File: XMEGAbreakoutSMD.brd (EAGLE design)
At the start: 160 x 100 mm, 23 parts, among them IC1 XMEGA16A4

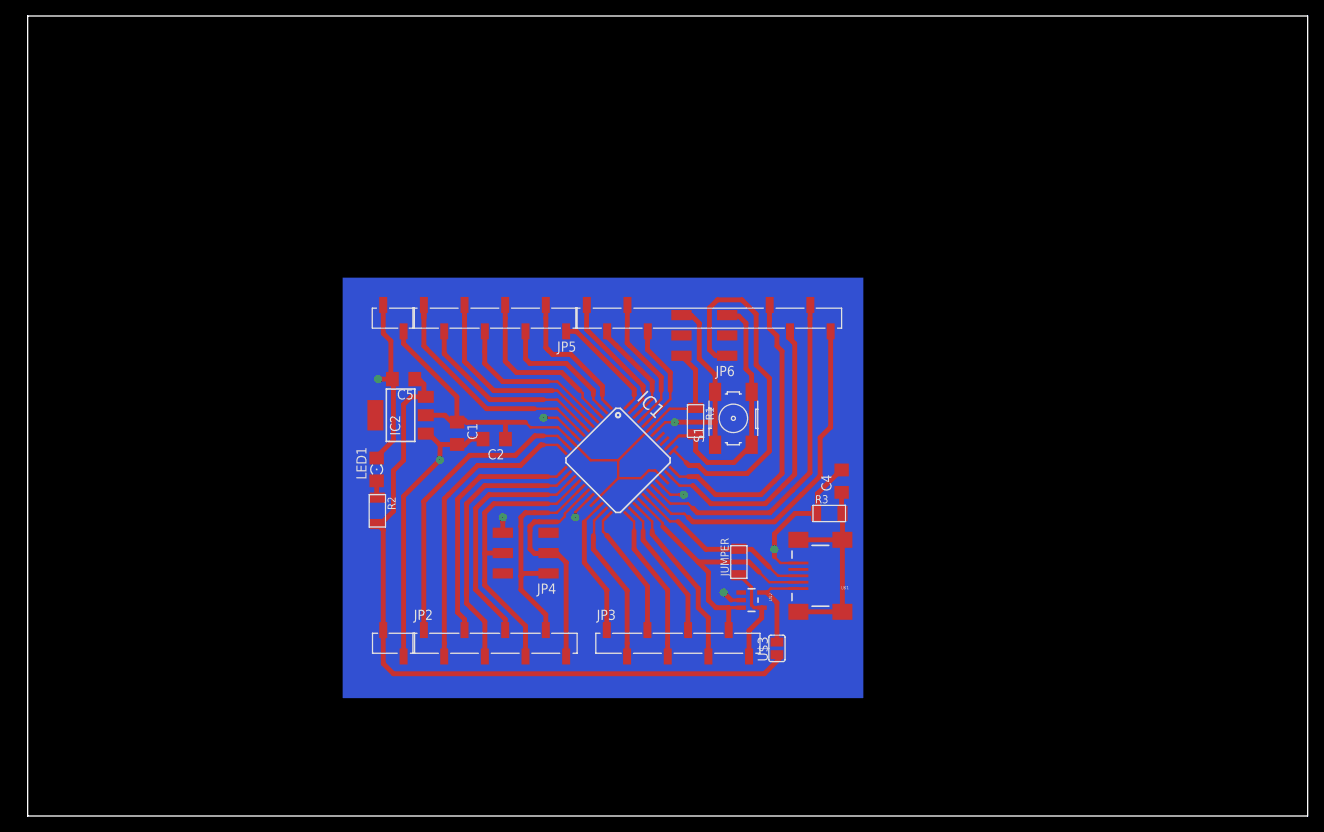
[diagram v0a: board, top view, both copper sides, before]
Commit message: smd
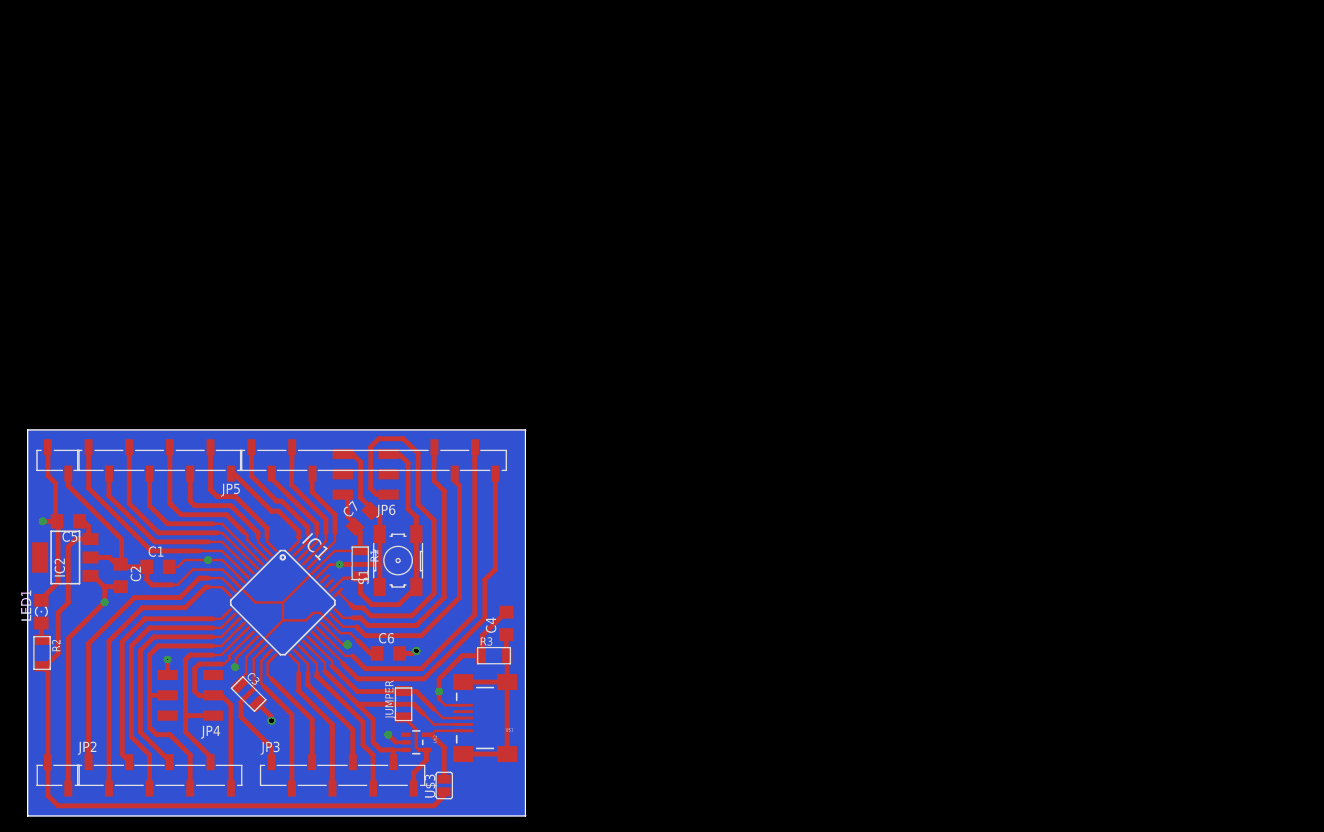
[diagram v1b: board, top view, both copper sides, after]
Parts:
- added C3: 0.1uF, fab:C1206FAB
- added C6, C7: 0.1uF, fab:C1206
- moved C2 49.7 mm to (11.6, 30.1), turned to 270 degrees
- moved JP6 45.8 mm to (42.3, 42.7)
- moved C4 45.5 mm to (59.8, 24.1)
- moved C5 45.5 mm to (5.08, 36.8)
- moved IC2 45.5 mm to (4.70, 32.3)
- moved JP4 45.5 mm to (20.3, 15.1)
- moved JUMPER 45.5 mm to (47.0, 14.0)
- moved LED1 45.5 mm to (1.71, 25.5)
- moved R1 45.5 mm to (41.6, 31.6)
- moved R2 45.5 mm to (1.80, 20.4)
- moved S1 45.5 mm to (46.3, 31.9)
- moved IC1 45.5 mm to (31.9, 26.7)
- moved JP1 45.5 mm to (58.5, 44.5)
- moved JP5 45.5 mm to (7.62, 44.5)
- moved JP8 45.5 mm to (2.54, 44.5)
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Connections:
- net GND: now also C3.2, C6.2, C7.2
- net VCC: now also C3.1, C6.1, C7.1
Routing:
- net GND: track 228.3 -> 261.4 mm, vias 9 -> 14
- net VCC: track 77.2 -> 90.5 mm
- net PE3: track 37.6 -> 34.7 mm
- net PE2: track 36.9 -> 34.4 mm
- net VBUS: track 102.8 -> 100.4 mm
- net N$13: track 34.6 -> 32.8 mm
- net N$23: track 20.6 -> 18.8 mm
- net N$9: track 30.9 -> 29.2 mm
- net PE0: track 43.7 -> 45.3 mm
- net PE1: track 43.6 -> 45.1 mm
- net N$16: track 37.9 -> 36.6 mm
- net MISO: track 28.0 -> 26.7 mm
- net SCK: track 28.7 -> 27.4 mm
- net N$12: track 30.2 -> 29.0 mm
- net N$14: track 31.3 -> 30.1 mm
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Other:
- board size 160 x 100 mm -> 62.2 x 48.3 mm
